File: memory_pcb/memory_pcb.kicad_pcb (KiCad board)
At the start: 2 copper layers, 100 x 50 mm, 55 parts, among them P1 AFC01-S10FCC-00, SW1 SW_Push, SW2 SW_Push, U1 AP3602AKTR-G1 SETUPUP, U10 DMG3415U, U11 SS54_C22452, U12 TYPE-C-31-M-12, U2 ESP32-S3-WROOM-1(N16R8), U3 100SP3T2B4M6RE, U4 TS-1088-AR02016, U5 BOOT, U6 MAX17048G+T10 FUEL GAUGE, U7 MCP73831T-2ACI/OT Charger, U8 S2B-PH-SM4-TB(LF)(SN)JST-PH C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, U9 AP2112K-3_3TRG1 Regulator

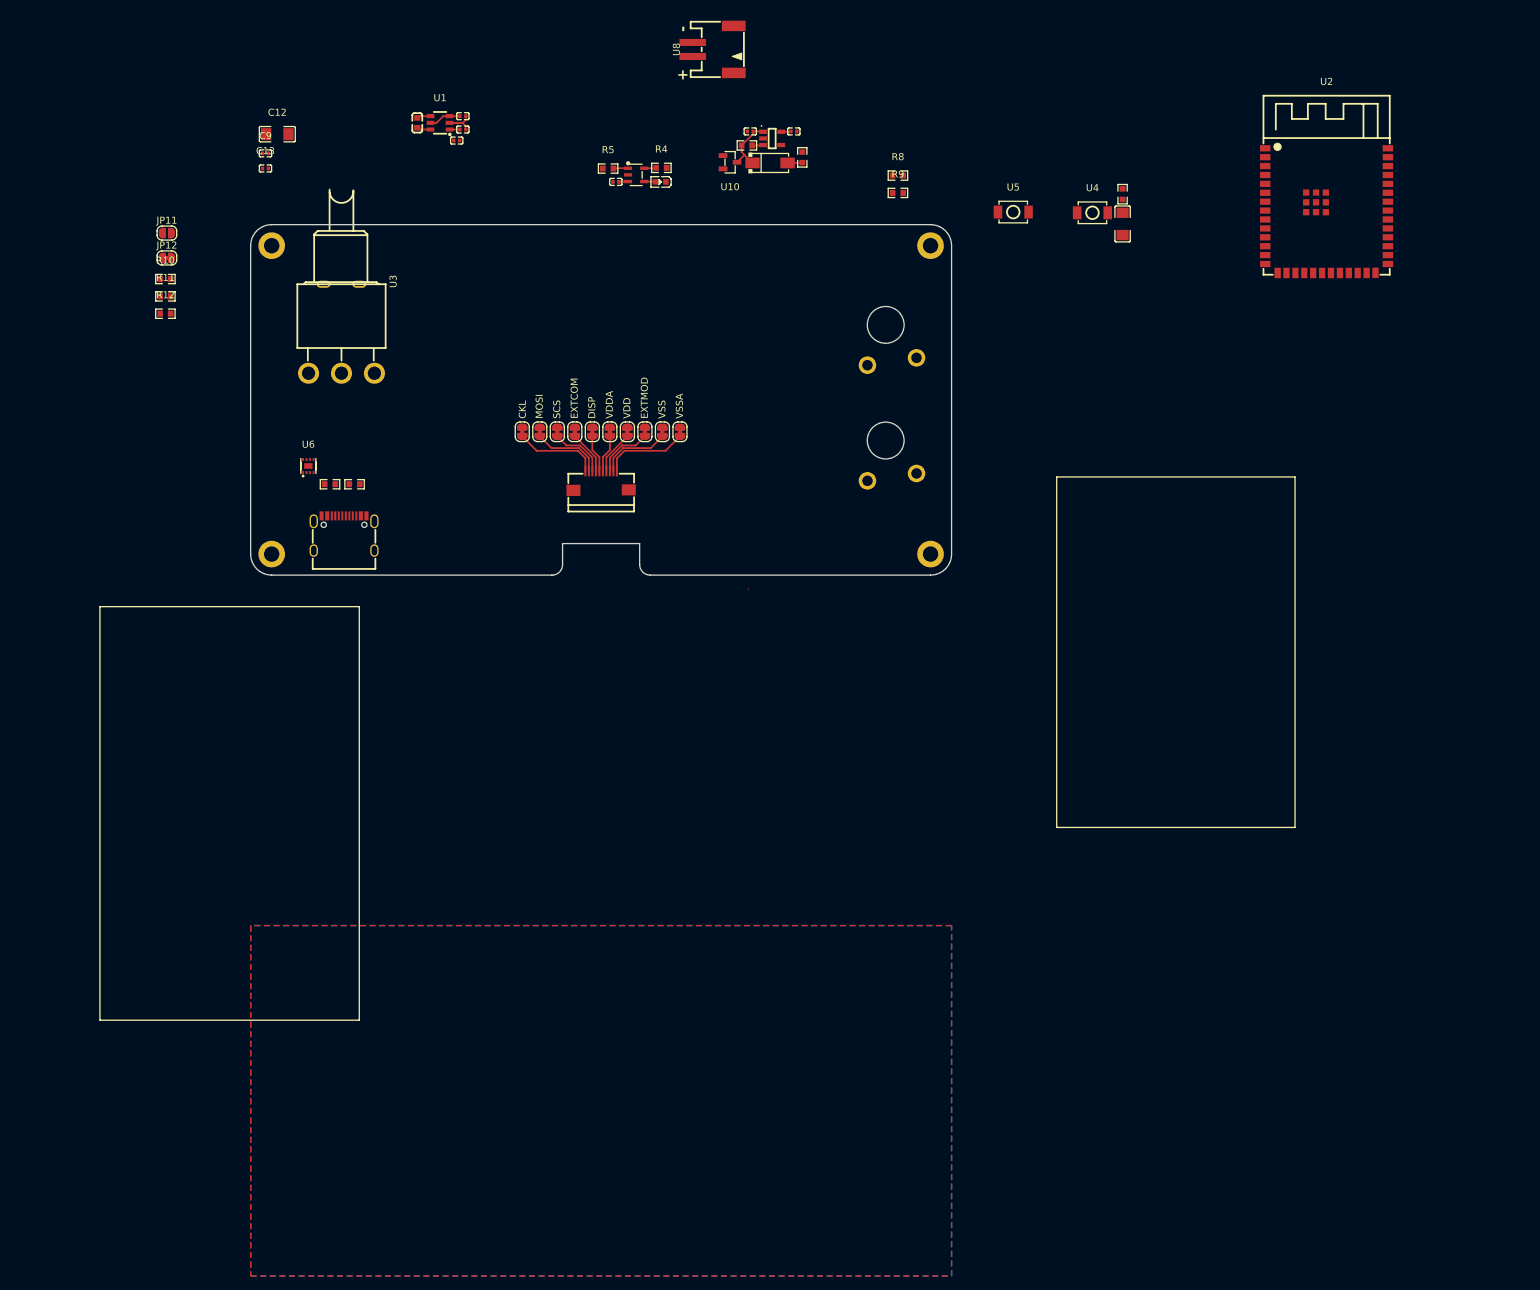
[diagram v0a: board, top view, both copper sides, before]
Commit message: and so it begins
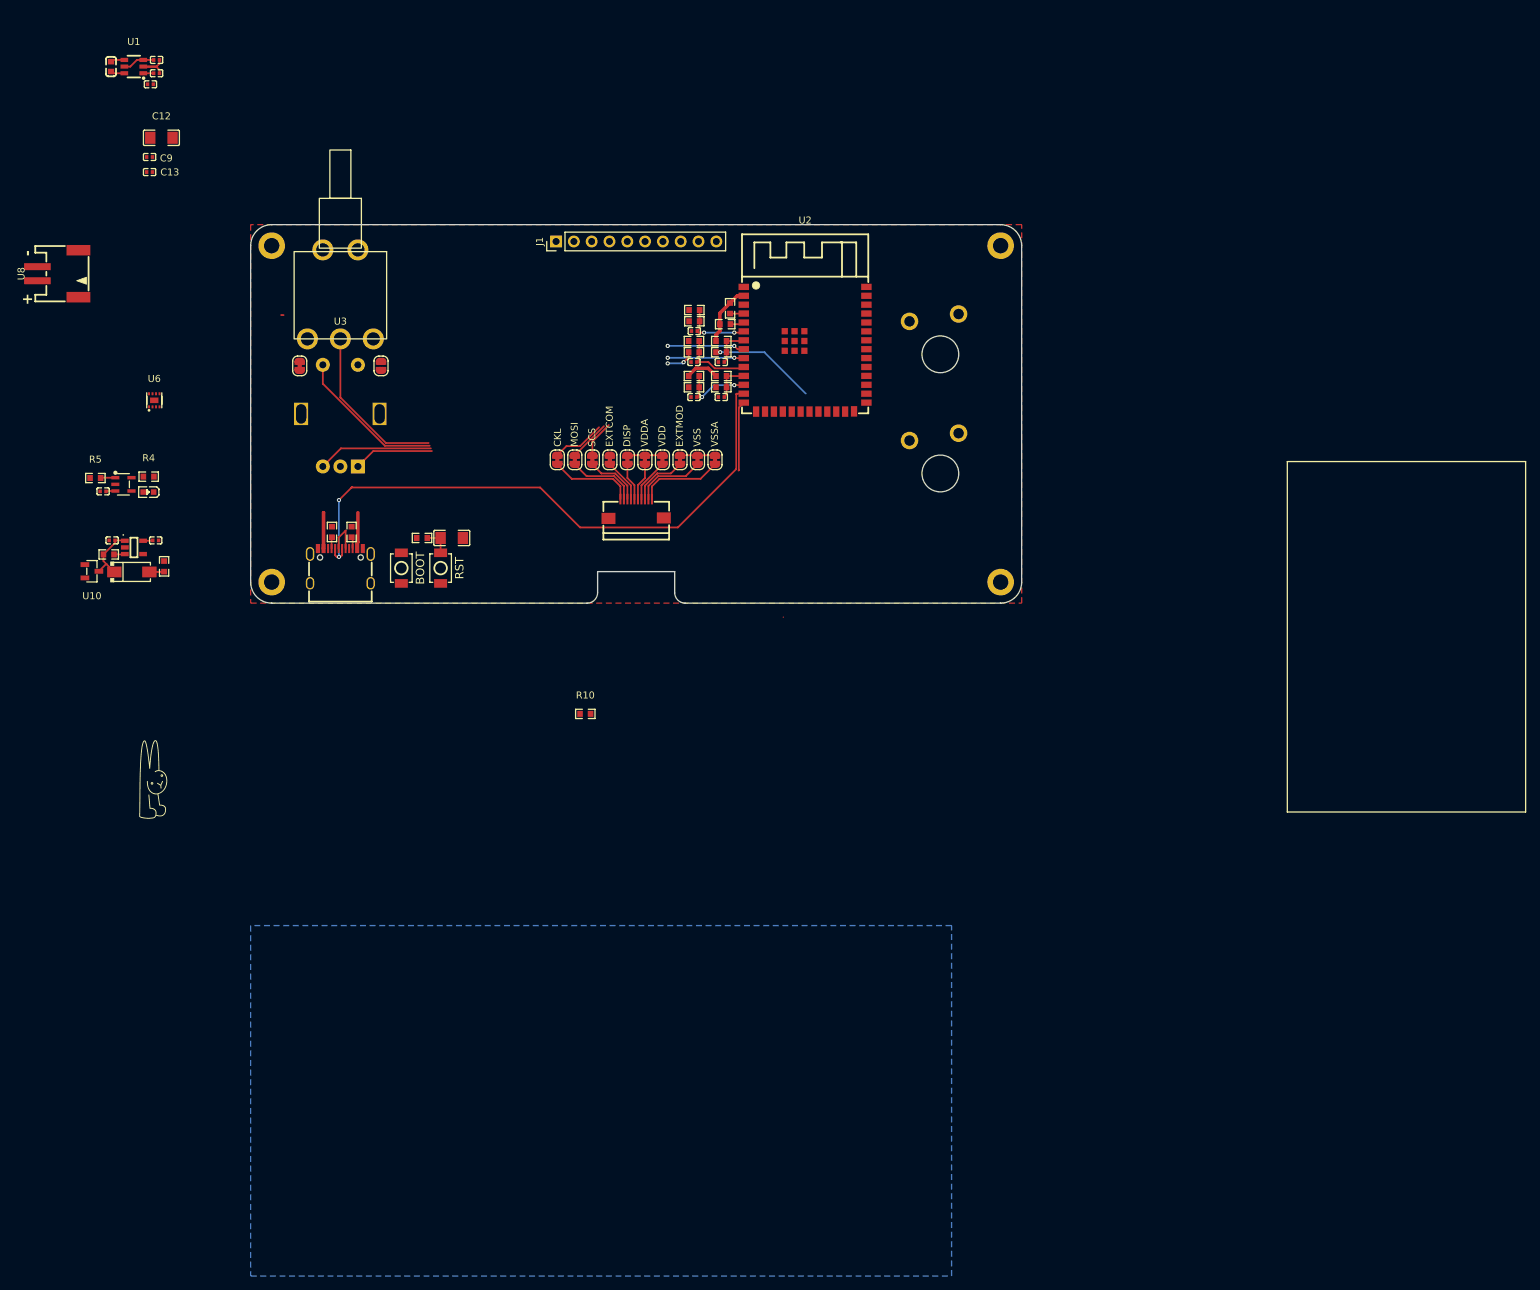
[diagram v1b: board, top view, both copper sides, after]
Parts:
- added C11: 0.1uF, new_lib_footprint:C0402, F.Cu at (113.3, 65.2)
- added C14: 0.1uF, new_lib_footprint:C0402, F.Cu at (113.2, 69.6)
- added C15: 0.1uF, new_lib_footprint:C0402, F.Cu at (117.1, 74.6)
- added C16: 0.1uF, new_lib_footprint:C0402, F.Cu at (113.2, 74.6)
- added C2: 0.1uF, new_lib_footprint:C0402, F.Cu at (117.1, 69.6)
- added ENC1: RotaryEncoder_Switch, Rotary_Encoder:RotaryEncoder_Alps_EC11E-Switch_Vertical_H20mm, B.Cu at (62.8, 77.0)
- added J1: Conn_01x10, Connector_PinHeader_2.54mm:PinHeader_1x10_P2.54mm_Vertical, F.Cu at (93.6, 52.4)
- added R13: 5.1kOhm, new_lib_footprint:R0603, F.Cu at (113.2, 71.6)
- added R14: 5.1kOhm, new_lib_footprint:R0603, F.Cu at (117.1, 71.6)
- added R15: 5.1kOhm, new_lib_footprint:R0603, F.Cu at (113.2, 66.6)
- added R16: 1kOhm, new_lib_footprint:R0603, F.Cu at (117.1, 68.2)
- added R17: 1kOhm, new_lib_footprint:R0603, F.Cu at (113.3, 63.8)
- added R18: 1kOhm, new_lib_footprint:R0603, F.Cu at (113.2, 68.2)
- added R19: 1kOhm, new_lib_footprint:R0603, F.Cu at (117.1, 73.2)
- added R20: 1kOhm, new_lib_footprint:R0603, F.Cu at (113.2, 73.2)
- U3: footprint new_lib_footprint:SW-TH_100SP3T2B4M6RE -> new_lib_footprint:MTS-102-C3
- moved R3 111.3 mm to (74.4, 94.7), turned to 180 degrees
- moved U9 108.1 mm to (33.4, 96.0)
- moved C7 108.1 mm to (30.2, 95.0)
- moved C8 108.1 mm to (36.5, 95.0)
- moved R6 108.1 mm to (29.8, 97.0)
- moved R7 108.1 mm to (37.7, 98.7)
- moved U11 108.1 mm to (33.1, 99.5)
- moved U10 108.1 mm to (27.4, 99.4)
- moved U4 105.9 mm to (77.1, 99.0), turned to 90 degrees
- moved C5 105.7 mm to (78.7, 94.7), turned to 180 degrees
- moved U5 101.0 mm to (71.5, 99.0), turned to 90 degrees
- moved U8 98.8 mm to (22.5, 57.0)
- moved R10 86.2 mm to (97.7, 119.8)
- moved R5 85.4 mm to (27.8, 86.2)
- moved U7 85.4 mm to (31.8, 87.1)
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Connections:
- SW1 pad 1: /BTN1 -> Net-(R17-Pad2)
- SW2 pad 1: /BTN2 -> Net-(R16-Pad2)
- U2 pad 10: unconnected-(U2-IO17-Pad10) -> /ENC_SIG_A
- U2 pad 11: unconnected-(U2-IO18-Pad11) -> /ENC_SIG_B
- U2 pad 12: unconnected-(U2-IO8-Pad12) -> /ENC_BTN
- U2 pad 15: /SDA -> unconnected-(U2-IO3-Pad15)
- U2 pad 23: unconnected-(U2-IO21-Pad23) -> /21
- U2 pad 24: unconnected-(U2-IO47-Pad24) -> /47
- U2 pad 25: unconnected-(U2-IO48-Pad25) -> /48
- U2 pad 38: unconnected-(U2-IO2-Pad38) -> /02
- U2 pad 39: unconnected-(U2-IO1-Pad39) -> /01
- U2 pad 4: /SCL -> /SDA
- U2 pad 5: unconnected-(U2-IO5-Pad5) -> /SCL
- U2 pad 6: unconnected-(U2-IO6-Pad6) -> /BTN1
- U2 pad 7: unconnected-(U2-IO7-Pad7) -> /BTN2
- U2 pad 8: unconnected-(U2-IO15-Pad8) -> /PWR_SW
- U2 pad 9: unconnected-(U2-IO16-Pad9) -> /ALRT
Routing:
- net /D-: track 0.00 -> 86.1 mm, vias 0 -> 2
- net /PWR_SW: track 0.00 -> 34.7 mm, vias 0 -> 2
- net Net-(ENC1-PadS1): track 0.00 -> 21.6 mm
- net Net-(ENC1-PadB): track 0.00 -> 16.5 mm
- net /D+: track 0.00 -> 15.5 mm
- net Net-(ENC1-PadA): track 0.00 -> 15.5 mm, vias 0 -> 2
- net Net-(R16-Pad2): track 0.00 -> 15.3 mm, vias 0 -> 1
- net +3.3V: track 5.97 -> 19.5 mm
- net /ALRT: track 0.00 -> 10.9 mm, vias 0 -> 2
- net /ENC_BTN: track 0.00 -> 10.5 mm, vias 0 -> 2
- net /ENC_SIG_A: track 0.00 -> 10.3 mm
- net /BTN1: track 0.00 -> 9.99 mm, vias 0 -> 2
- net VBUS: track 3.73 -> 12.5 mm
- net /CLK: track 0.00 -> 7.60 mm
- net /MOSI: track 0.00 -> 5.87 mm
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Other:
- board size 100 x 50 mm -> 110 x 54 mm
- board text added: "BOOT"
- board text added: "RST"
